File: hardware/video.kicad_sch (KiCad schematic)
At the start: 11 parts, among them J6 DE15_Socket_HighDensity, U13 V9958, U14 74AUC2G32, U15 41464, U16 41464, U17 41464, U18 41464, U19 SN74LVC245APW, U21 LM1881, U22 74LVC1G07, Y3 TFT680

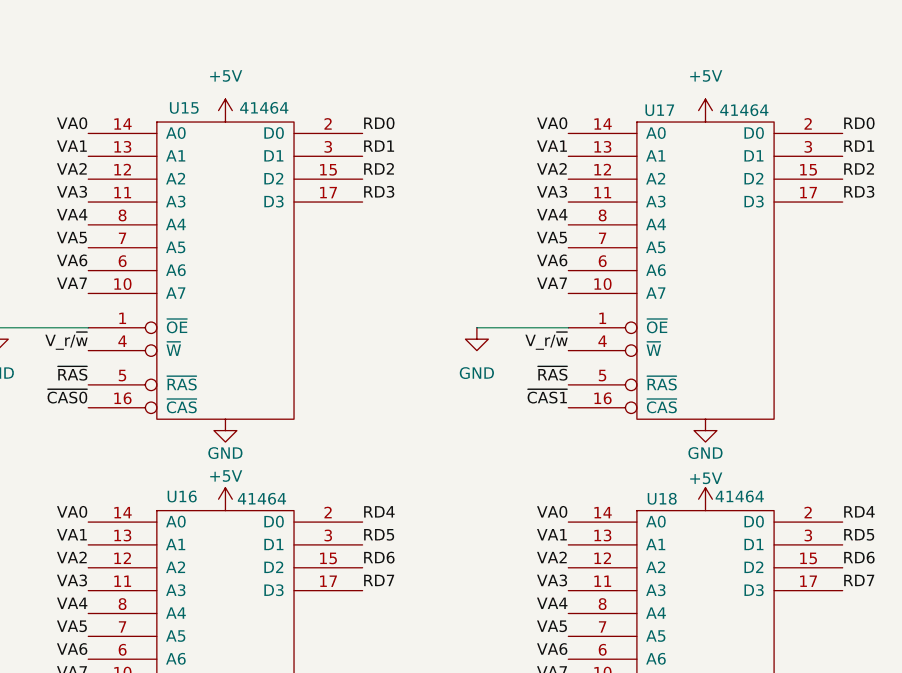
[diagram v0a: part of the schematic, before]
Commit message: Minor Improvemnts
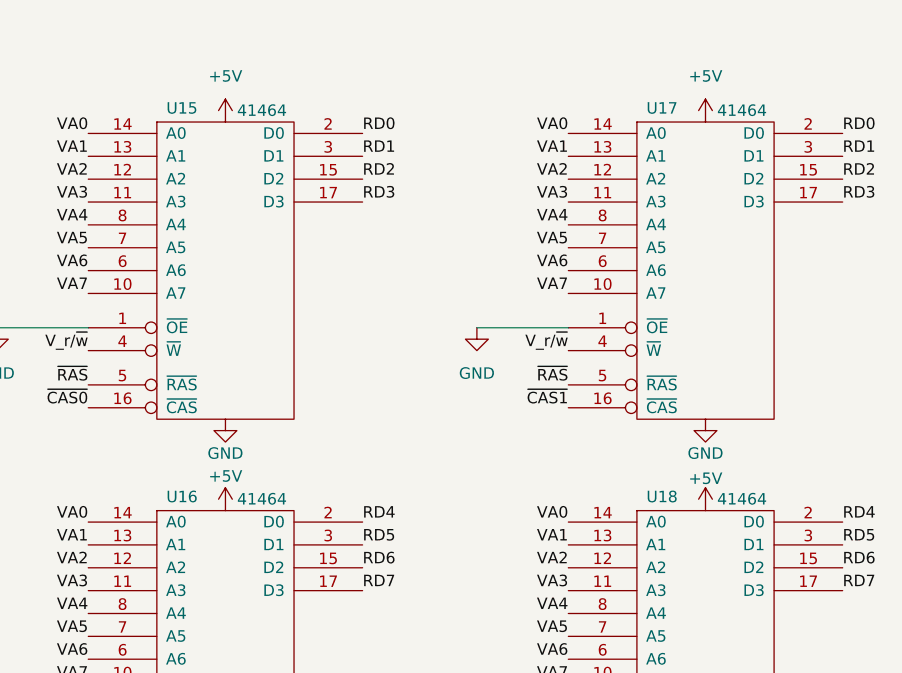
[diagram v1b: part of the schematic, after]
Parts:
- J6: footprint (none) -> Connector_Dsub:DSUB-15_Socket_Horizontal_P2.77x2.84mm_EdgePinOffset9.40mm
- U14: footprint (none) -> Package_SO:SSOP-8_2.95x2.8mm_P0.65mm
- U15, U16, U17, U18: footprint (none) -> Package_DIP:DIP-18_W7.62mm
- U21: footprint (none) -> Package_DIP:DIP-8_W7.62mm
- U22: footprint (none) -> Package_TO_SOT_SMD:SOT-23-5
